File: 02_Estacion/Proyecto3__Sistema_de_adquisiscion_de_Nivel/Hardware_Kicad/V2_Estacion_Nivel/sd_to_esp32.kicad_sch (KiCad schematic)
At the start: 9 parts, among them J1 Micro_SD_Card_Det1

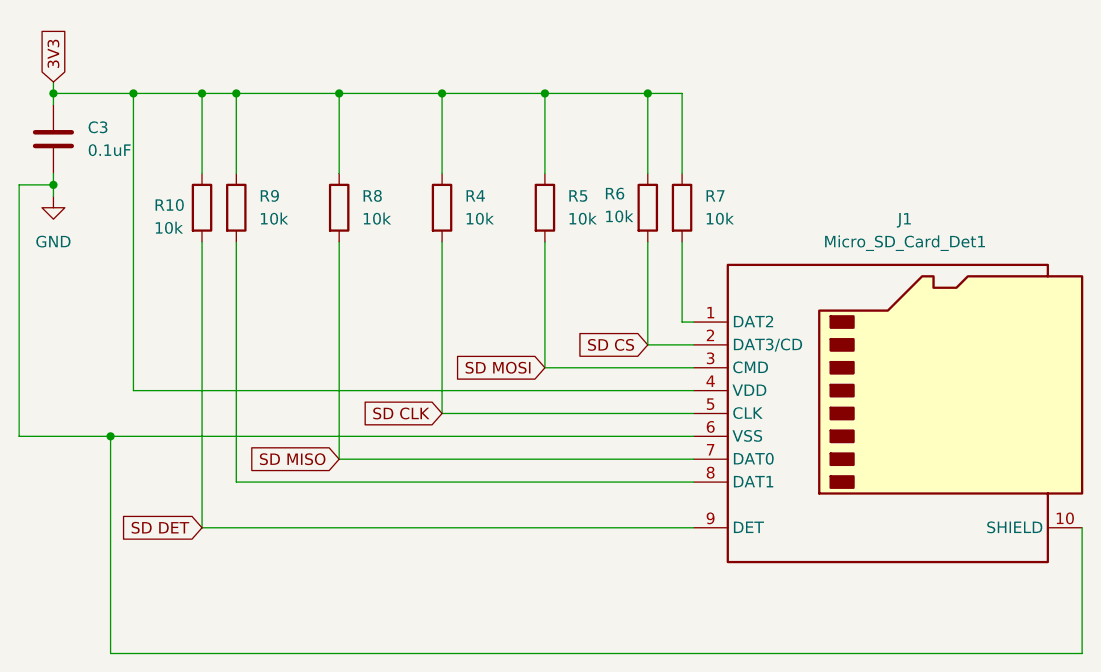
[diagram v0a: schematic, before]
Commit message: update
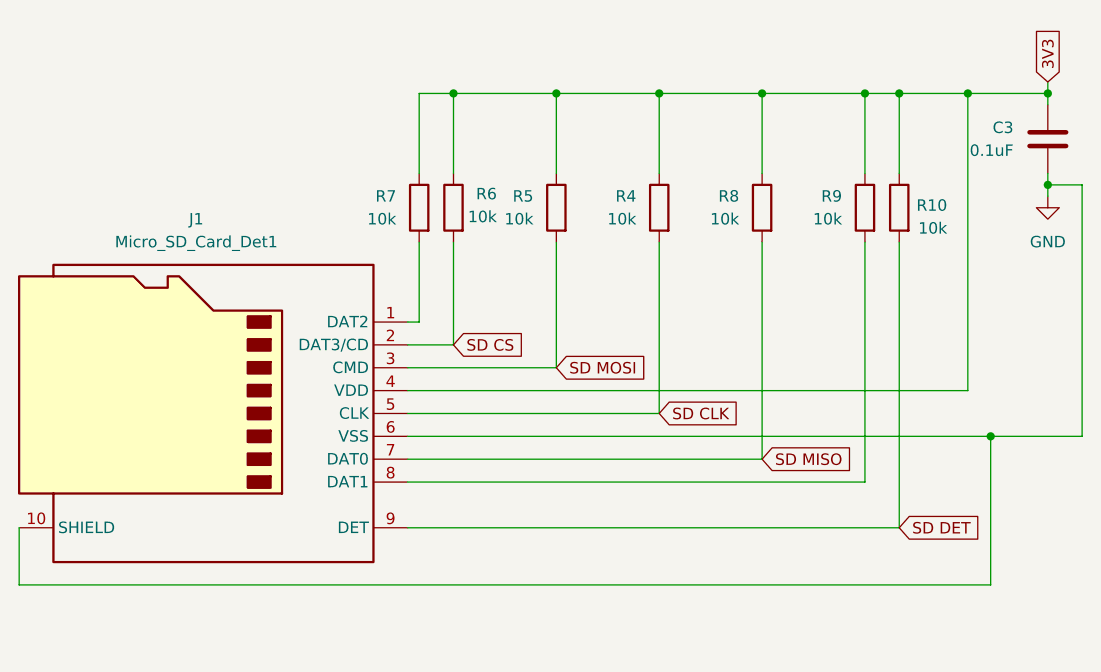
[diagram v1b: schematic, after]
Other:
- moved on the sheet: C3, J1, R10, R4, R5, R6, R7, R8, R9
